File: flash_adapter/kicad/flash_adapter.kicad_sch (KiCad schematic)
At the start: 7 parts, among them J1 Conn_01x10, J2 Conn_01x10, J3 DS1044-160G, SW1 MK-12C02-G020

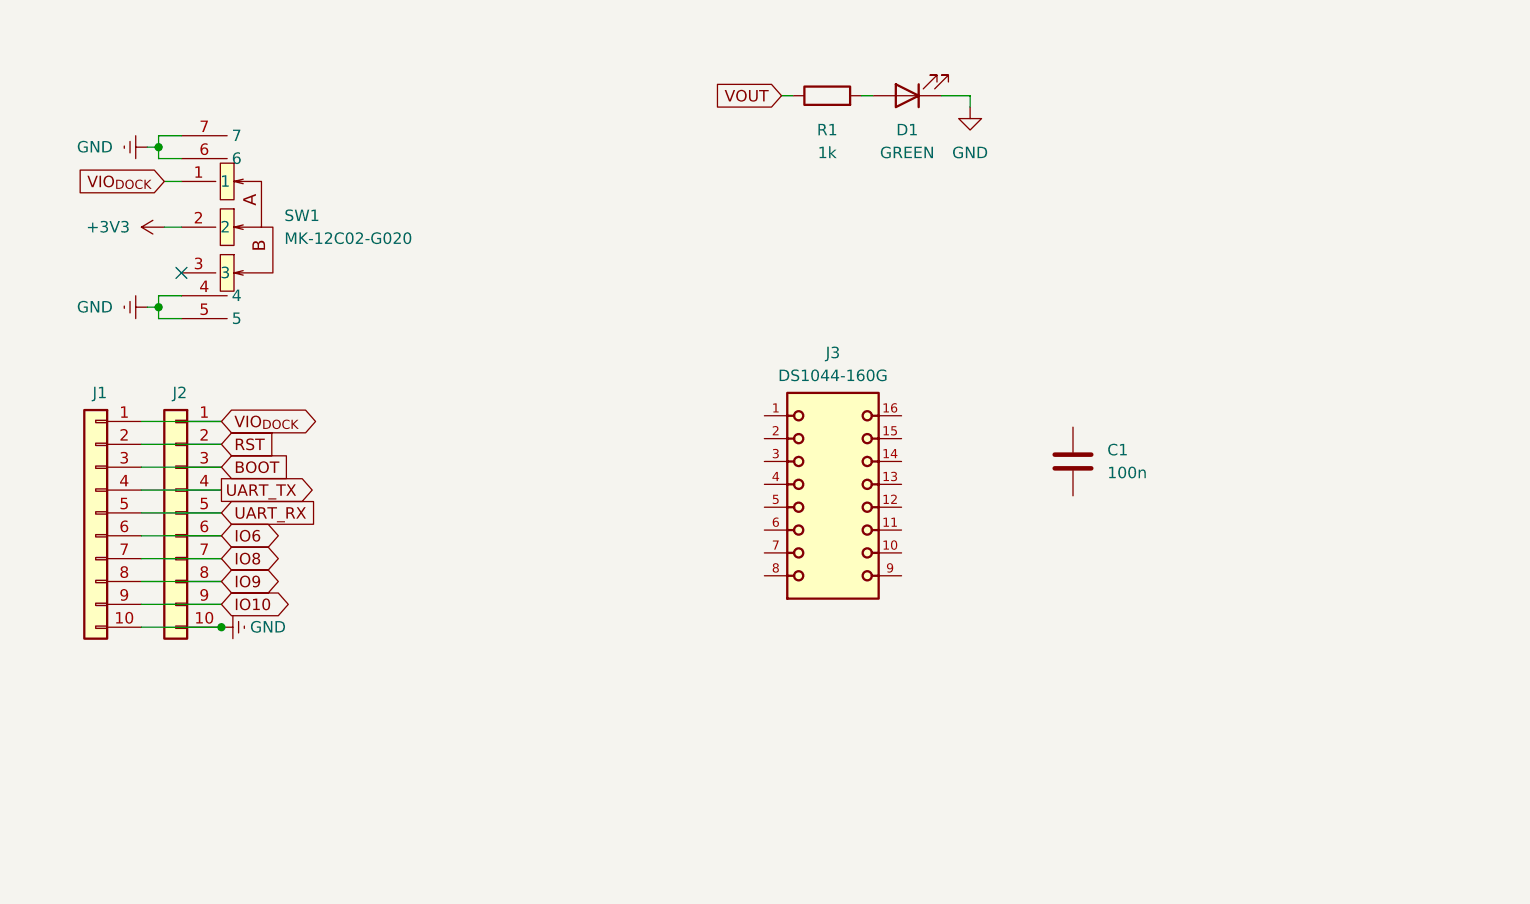
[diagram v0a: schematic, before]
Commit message: Updated flash adapter
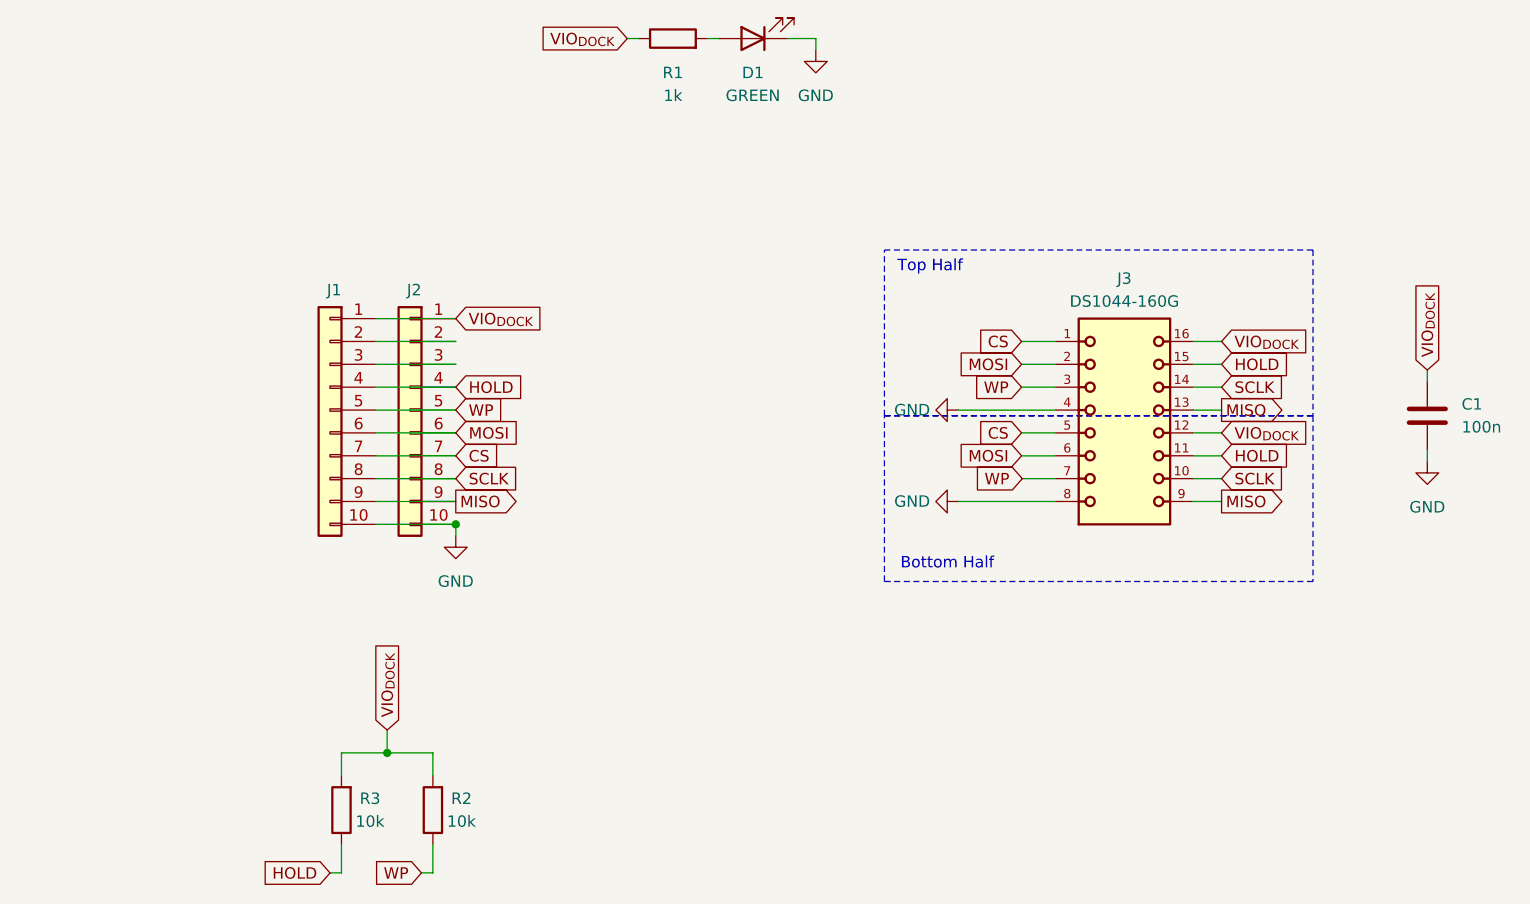
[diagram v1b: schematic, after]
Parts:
- removed SW1: MK-12C02-G020, C5-Addon:SW-SMD_MK-12C02-G020, symbol C5-Addon:MK-12C02-G020
- added R2, R3: 10k, Resistor_SMD:R_0805_2012Metric, symbol Device:R
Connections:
- net IO10 is gone; now on net MISO: J1.9 (Pin_9), J2.9 (Pin_9)
- net IO6 is gone; now on net MOSI: J1.6 (Pin_6), J2.6 (Pin_6)
- net IO8 is gone; now on net CS: J1.7 (Pin_7), J2.7 (Pin_7)
- net IO9 is gone; now on net SCLK: J1.8 (Pin_8), J2.8 (Pin_8)
- net UART_RX is gone; now on net WP: J1.5 (Pin_5), J2.5 (Pin_5)
- net UART_TX is gone; now on net HOLD: J1.4 (Pin_4), J2.4 (Pin_4)
- net VOUT is gone; now on net VIO_{DOCK}: R1.1
- net GND: now also C1.2, J3.4, J3.8
- net VIO_{DOCK}: now also C1.1, J3.12, J3.16, R2.2, R3.2
- net CS: now reaches J3.1
- net CS: now also J3.5
- net SCLK: now reaches J3.10
- net SCLK: now also J3.14
- net HOLD: now reaches J3.11
- net HOLD: now also J3.15, R3.1
- net MISO: now reaches J3.13
- net MISO: now also J3.9
- net MOSI: now reaches J3.2
- net MOSI: now also J3.6
- net WP: now reaches J3.3
- net WP: now also J3.7, R2.1
- net BOOT: no longer names the net of J1.3 (Pin_3), J2.3 (Pin_3)
- net RST: no longer names the net of J1.2 (Pin_2), J2.2 (Pin_2)
- no-connect marks 1 -> 0
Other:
- note added: "Bottom Half"
- note added: "Top Half"
- moved on the sheet: C1, D1, J1, J2, J3, R1
